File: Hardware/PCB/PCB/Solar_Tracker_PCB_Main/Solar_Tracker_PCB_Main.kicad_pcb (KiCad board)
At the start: 4 copper layers, 94 x 96.5 mm, 66 parts, among them IC1 ESP32-S3-WROOM-1-N4R8, IC2 TPS54302DDCT, IC3 BNO085, IC4 PCF2131TFY, IC6 TLV76133DCYR, J1 SM08B-SRSS-TB_LF__SN_, J2 USB4940-00-A, J3 Conn_01x06_Pin, J4 1977223-1, J5 1977223-1, J7 TB002-500-02BE, J8 SM08B-SRSS-TB_LF__SN_, J9 SM08B-SRSS-TB_LF__SN_, Q1 DMP2045U-7, Q2 DMP2045U-7, Y1 32.768kHz

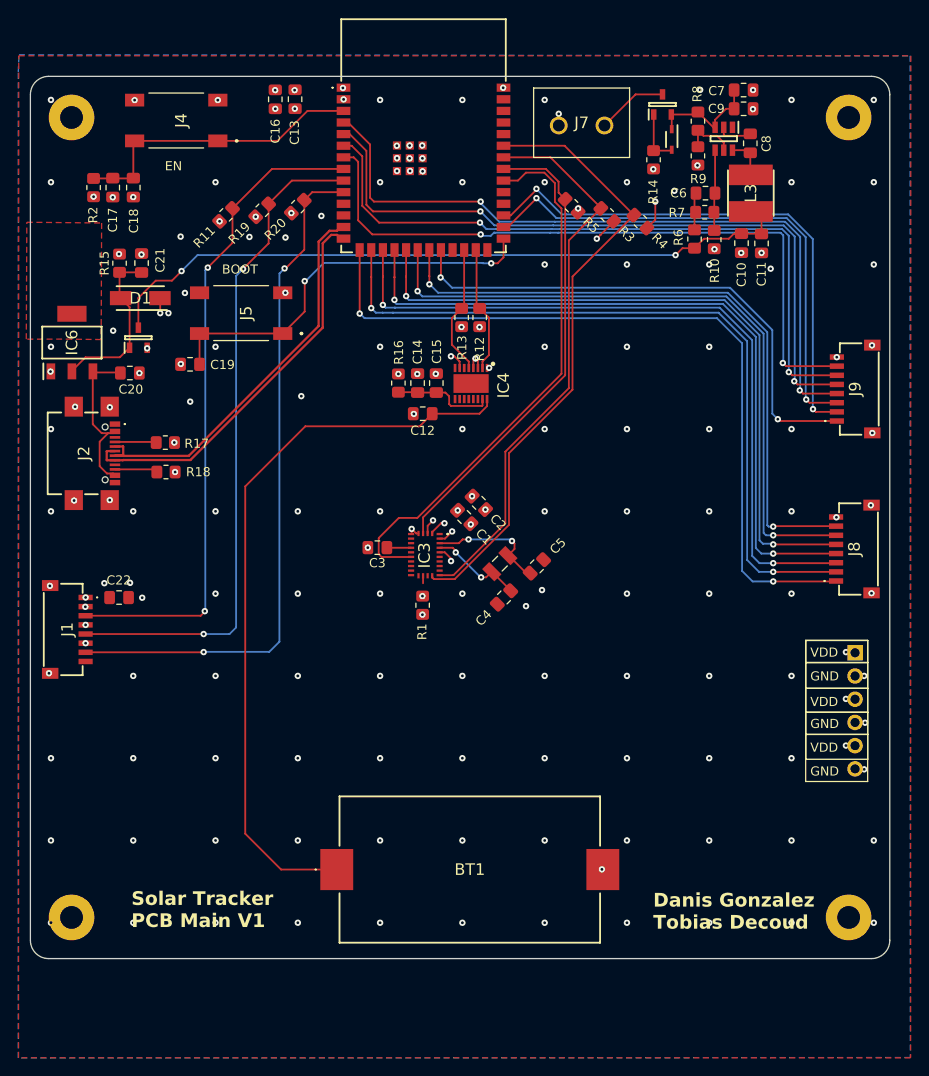
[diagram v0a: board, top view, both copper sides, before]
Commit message: cambios pcb main
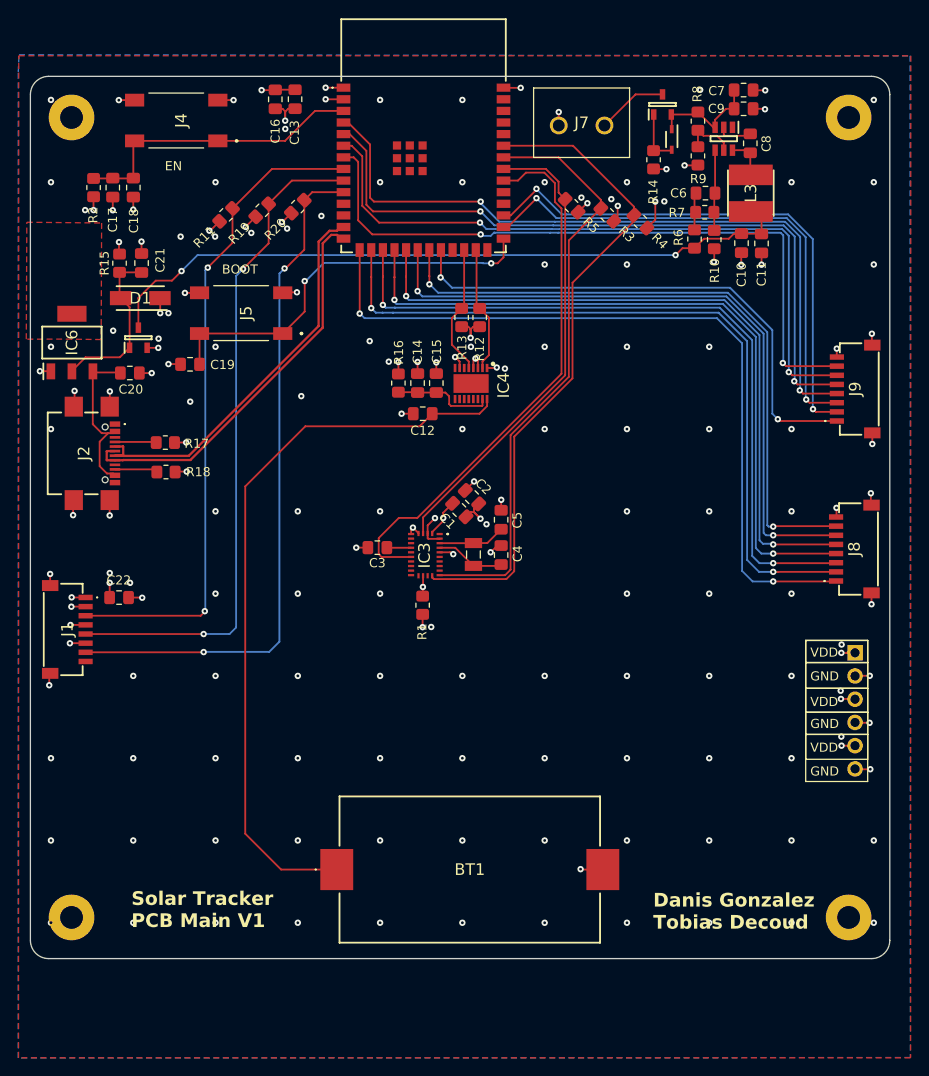
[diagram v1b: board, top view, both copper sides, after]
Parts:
- moved C5 6.43 mm to (123.0, 93.0), turned to 90 degrees
- moved C4 4.65 mm to (123.0, 96.9), turned to 90 degrees
- moved Y1 3.06 mm to (120.0, 96.8), turned to -90 degrees
- moved C2 0.97 mm to (119.8, 90.5)
- moved C1 0.93 mm to (118.4, 91.9)
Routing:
- net GND: track 11.8 -> 90.1 mm, vias 167 -> 163
- net VDD: track 13.5 -> 45.5 mm, vias 25 -> 22
- net /IMU/X_IN: track 13.4 -> 7.36 mm, vias 2 -> 0
- net IMU_SCL: track 68.1 -> 71.9 mm
- net IMU_SDA: track 61.3 -> 65.1 mm
- net /IMU/X_OUT: track 10.6 -> 7.61 mm, vias 3 -> 0
